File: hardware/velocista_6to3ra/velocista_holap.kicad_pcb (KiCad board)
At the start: 2 copper layers, 14 parts, among them J1 ENTRADA, J2 BORNERA_MOTOR_A, J3 BORNERA_MOTOR_B, J5 SENSORES_DE_PISO, SW1 SW_DE_ARRANQUE, U1 LM7805_TO220, U2 INTEGRADO_L293D

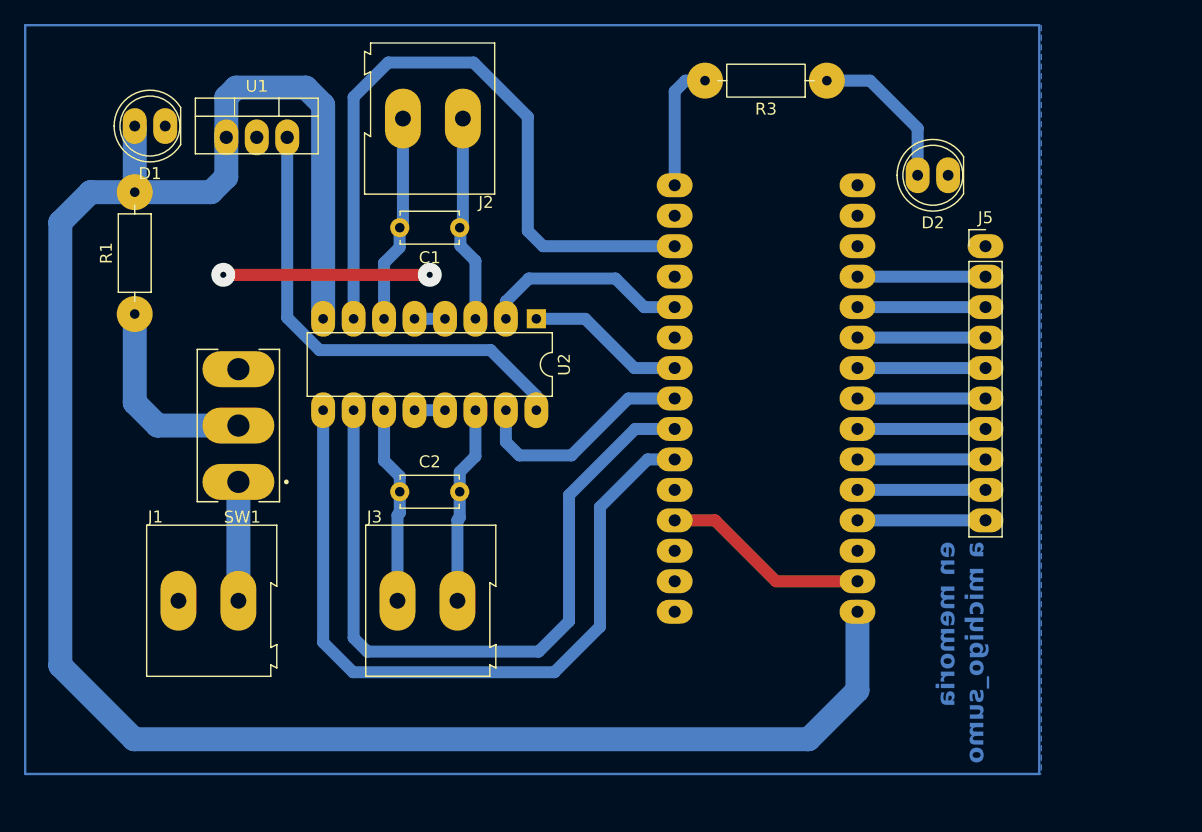
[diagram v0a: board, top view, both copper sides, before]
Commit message: 29/10_2
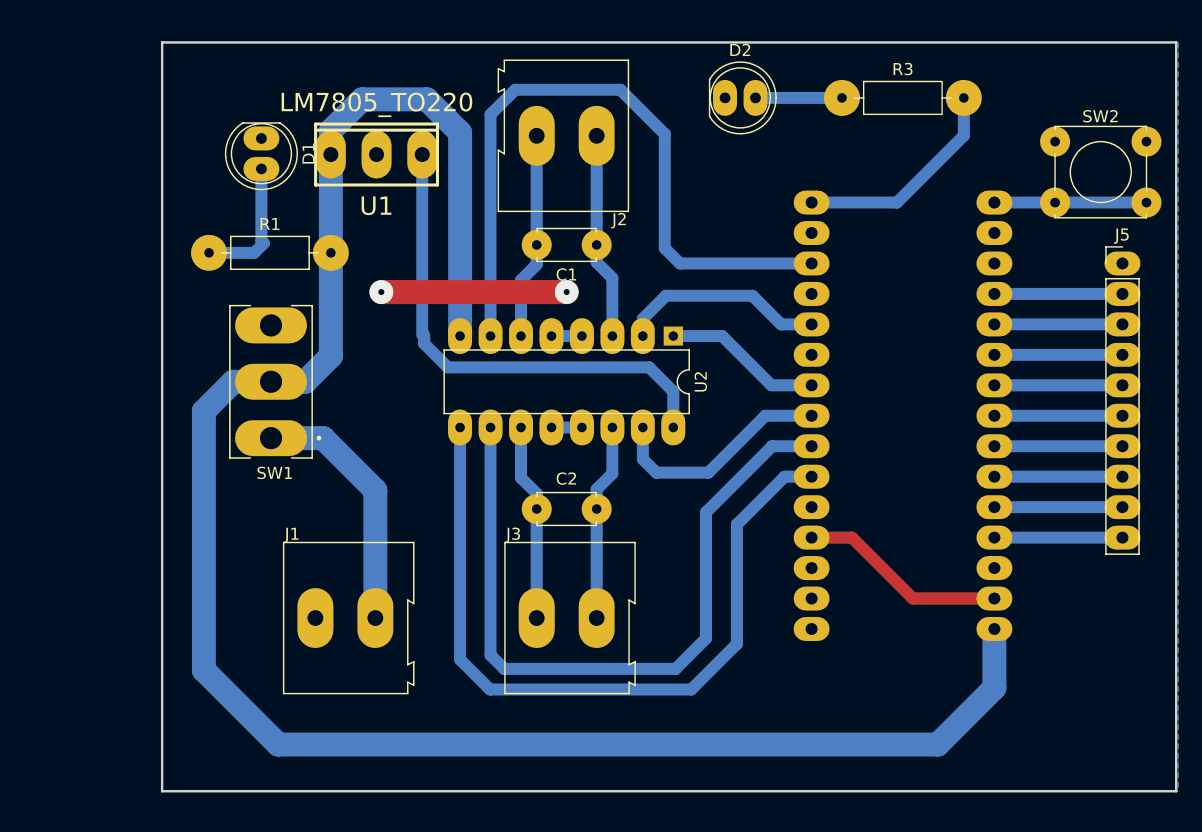
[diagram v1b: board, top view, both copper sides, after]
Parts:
- added SW2: SW_DE_ARRANQUE, Button_Switch_THT:SW_Tactile_Straight_KSA0Axx1LFTR, F.Cu at (161.2, 47.3)
- U1: footprint Package_TO_SOT_THT:TO-220-3_Vertical -> EESTN5:TO-220-2
- moved D2 19.7 mm to (133.7, 43.7), turned to 0 degrees
- moved U1 12.6 mm to (104.6, 48.4)
- moved J3 11.7 mm to (118.0, 87.0)
- moved J5 11.5 mm to (166.8, 57.5)
- moved C1 11.5 mm to (123.0, 55.9)
- moved C2 11.5 mm to (118.0, 78.0)
- moved J1 11.5 mm to (99.5, 87.0)
- moved U2 11.5 mm to (129.3, 63.5)
- moved A1 11.5 mm to (140.9, 88.0)
- moved J2 11.2 mm to (123.0, 46.8)
- moved D1 8.09 mm to (95.0, 47.1), turned to -90 degrees
- moved R1 8.02 mm to (90.6, 56.6), turned to 0 degrees
- moved SW1 4.55 mm to (95.8, 67.3)
- moved R3 1.91 mm to (143.4, 43.7), turned to 0 degrees
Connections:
- A1 pad 12: pwm_motor_B -> unconnected-(A1-D9-Pad12)
- A1 pad 16: unconnected-(A1-D13-Pad16) -> Net-(A1-D13)
- D1 pad 2: VCC -> Net-(D1-A)
- R1 pad 1: Net-(SW1-B) -> Net-(D1-A)
- SW1 pad 2: Net-(SW1-B) -> VCC
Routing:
- net Net-(SW1-B): track 16.8 -> 0.00 mm
- net Net-(A1-D13): track 0.00 -> 12.7 mm
- net Net-(J1-Pin_2): track 9.91 -> 21.2 mm
- net Net-(D1-A): track 0.00 -> 11.2 mm
- net VCC: track 168.6 -> 158.2 mm
- net Net-(A1-D12): track 10.7 -> 18.1 mm
- net Net-(D2-A): track 13.1 -> 7.21 mm
- net GND: track 39.8 -> 37.9 mm
- net +5V: track 39.7 -> 41.2 mm
- net Motor_A_2: track 58.4 -> 57.7 mm
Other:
- board outline added: 84.6 x 62.4 mm
- board text removed: "en memoria a michigo_sumo"
